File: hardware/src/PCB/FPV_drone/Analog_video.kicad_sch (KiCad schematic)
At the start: 17 parts, among them J3 Conn_01x06, J5 JST_1mm_4, J6 JST_1mm_4, U2 AT7456ELAH_C42388749, Y2 ABM3B-27.000MHZ-10-B-1-U-T

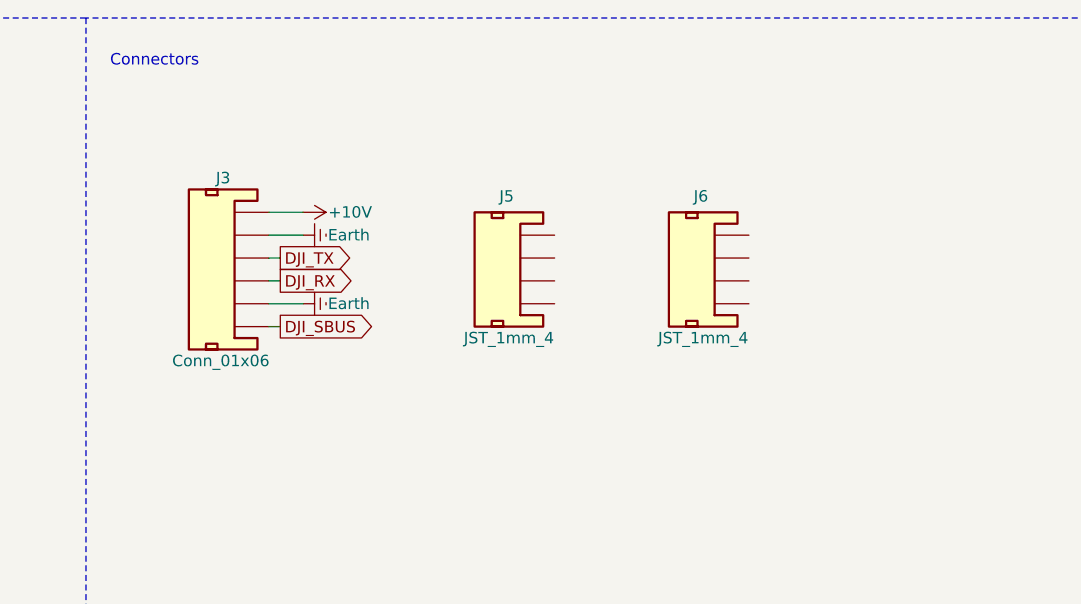
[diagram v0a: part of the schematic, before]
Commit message: update: schem finished
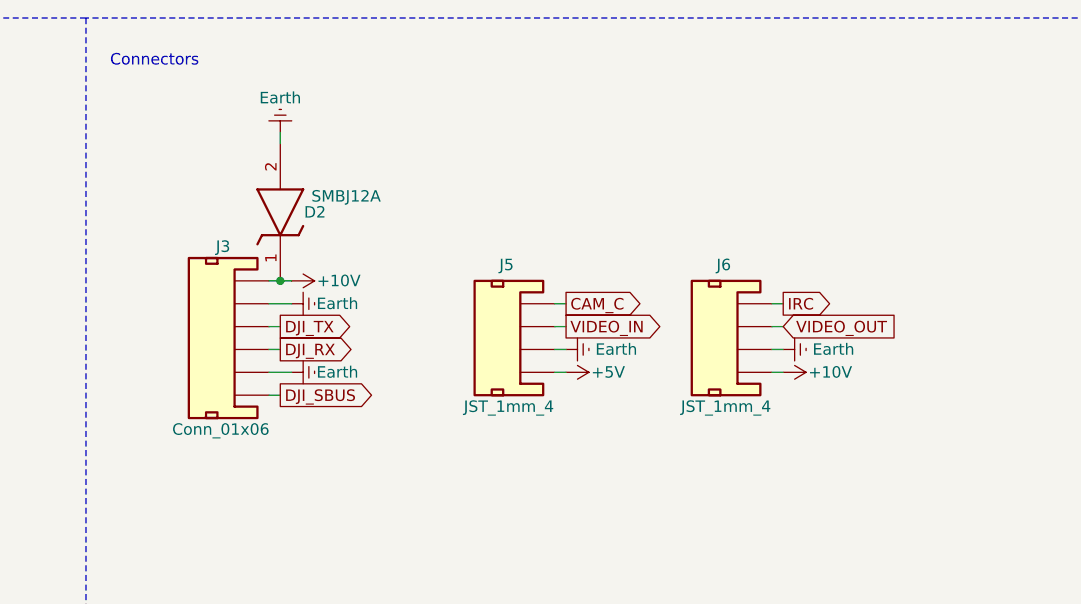
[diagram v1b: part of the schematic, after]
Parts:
- added D2: SMBJ12A, LIB:DIONM5436X261N, symbol lib:SMBJ12A
- U2: footprint (none) -> LIB:AT7456ELAH
- Y2: footprint ABM3B -> LIB:ABM3B
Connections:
- net +10V: now also J6.1, D2.1 (K)
- net Earth: now also J5.2, J6.2, D2.2 (A)
- net VIDEO_IN: now also J5.3
- net VIDEO_OUT: now also J6.3
- net +5V: now reaches J5.1
- net CAM_C: now reaches J5.4
- net IRC: now reaches J6.4
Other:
- moved on the sheet: J3, J5, J6
